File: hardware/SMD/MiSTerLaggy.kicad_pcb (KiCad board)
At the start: 2 copper layers, 19.8 x 12.5 mm, 9 parts, among them J1 USB_C_Receptacle_USB2.0, Q1 Q_Photo_NPN

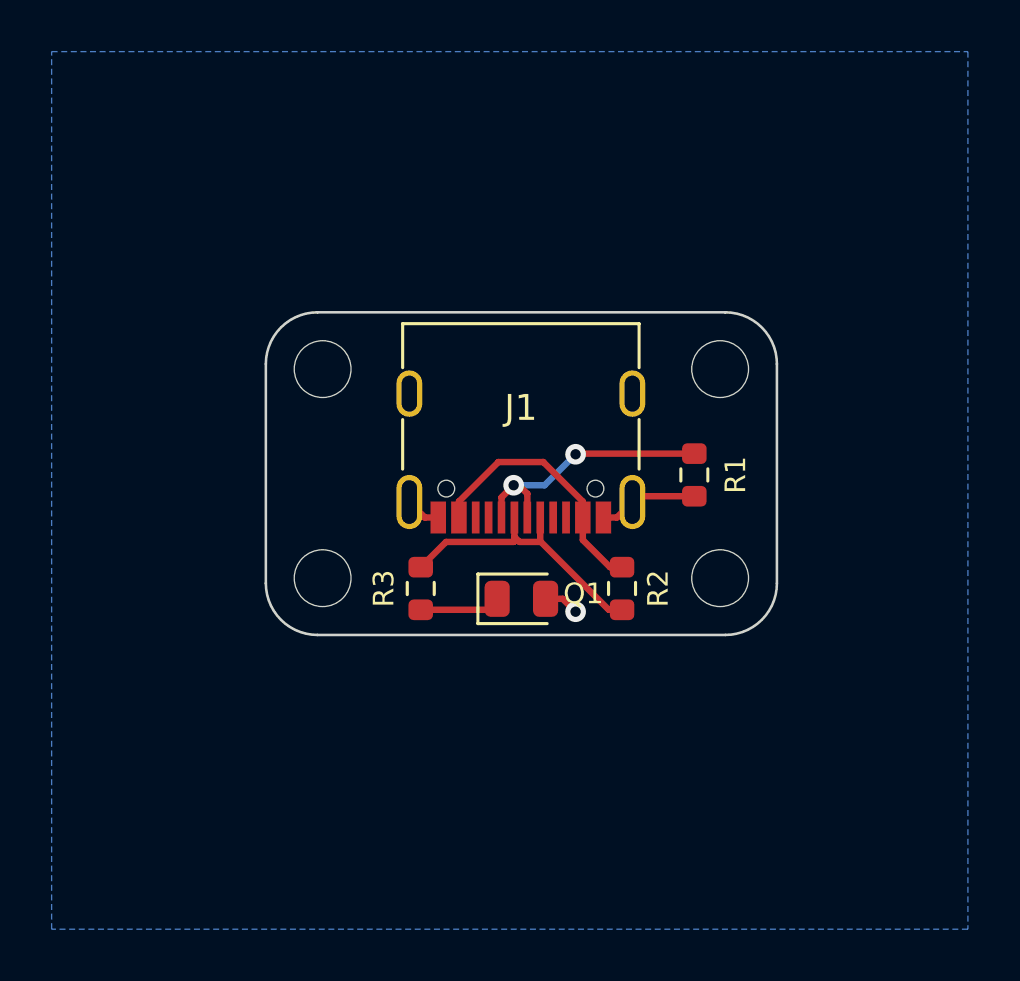
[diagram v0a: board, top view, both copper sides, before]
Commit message: New circuit design
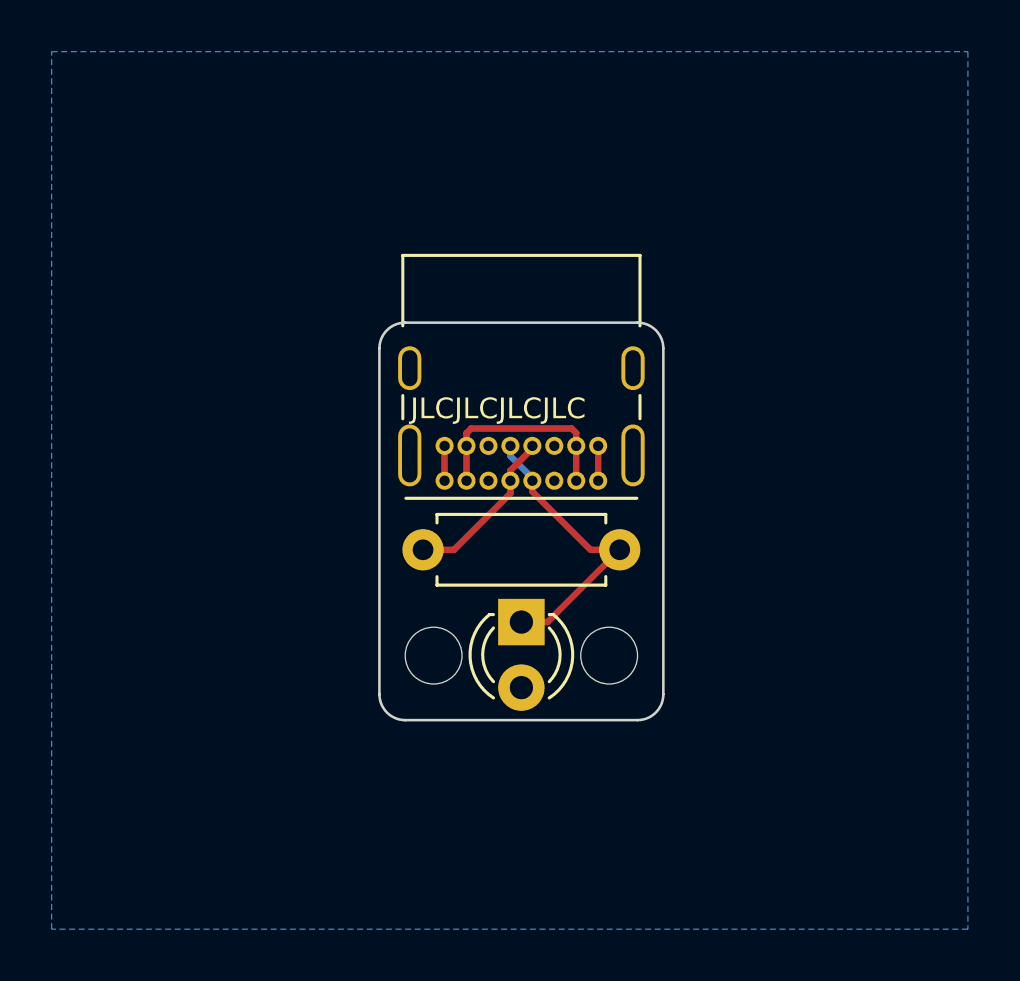
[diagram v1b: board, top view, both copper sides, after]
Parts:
- removed H3, H4: MountingHole_Pad, MountingHole:MountingHole_2.2mm_M2_ISO7380
- removed the R1 at (134.4, 73.4)
- removed R2: ??, Resistor_SMD:R_0603_1608Metric
- J1: footprint Connector_USB:USB_C_Receptacle_G-Switch_GT-USB-7010ASV -> Connector_USB:USB_C_Receptacle_GCT_USB4085
- Q1: value Q_Photo_NPN -> PT17-21C/L41/TR8; footprint LED_SMD:LED_0805_2012Metric -> LED_THT:LED_D3.0mm
- R1: renamed from R3; value ?? -> 750K; footprint Resistor_SMD:R_0603_1608Metric -> Resistor_THT:R_Axial_DIN0207_L6.3mm_D2.5mm_P7.62mm_Horizontal
- moved H2 11.9 mm to (131.1, 80.4)
- moved H1 11.9 mm to (124.3, 80.4)
- moved R1 7.85 mm to (131.5, 76.3), turned to 180 degrees
- moved J1 3.78 mm to (130.7, 73.6)
- moved Q1 0.90 mm to (127.7, 79.1), turned to -90 degrees
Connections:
- net Net-(J1-D--PadA7) renamed +3.3V
- J1 pad A4: +5V -> unconnected-(J1-VBUS-PadA4)
- J1 pad A6: Net-(J1-D+-PadA6) -> Net-(Q1-C)
- J1 pad A9: +5V -> unconnected-(J1-VBUS-PadA4)
- J1 pad B4: +5V -> unconnected-(J1-VBUS-PadA4)
- J1 pad B6: Net-(J1-D+-PadA6) -> Net-(Q1-C)
- J1 pad B9: +5V -> unconnected-(J1-VBUS-PadA4)
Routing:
- net Net-(J1-D+-PadA6): track 10.5 -> 0.00 mm, vias 2 -> 0
- net +5V: track 10.1 -> 0.00 mm
- net Net-(Q1-C): track 3.14 -> 11.4 mm
- net unconnected-(J1-VBUS-PadA4): track 0.00 -> 8.09 mm
- net +3.3V: track 11.2 -> 6.49 mm
- net GND: track 6.60 -> 2.70 mm, vias 1 -> 0
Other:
- board size 19.8 x 12.5 mm -> 11 x 15.4 mm
- board text added: "@wickerwaka"
- board text added: "JLCJLCJLCJLC"
- board text added: "MrLaggy"
- board text added: "v1.0"

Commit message: MOSFET usage
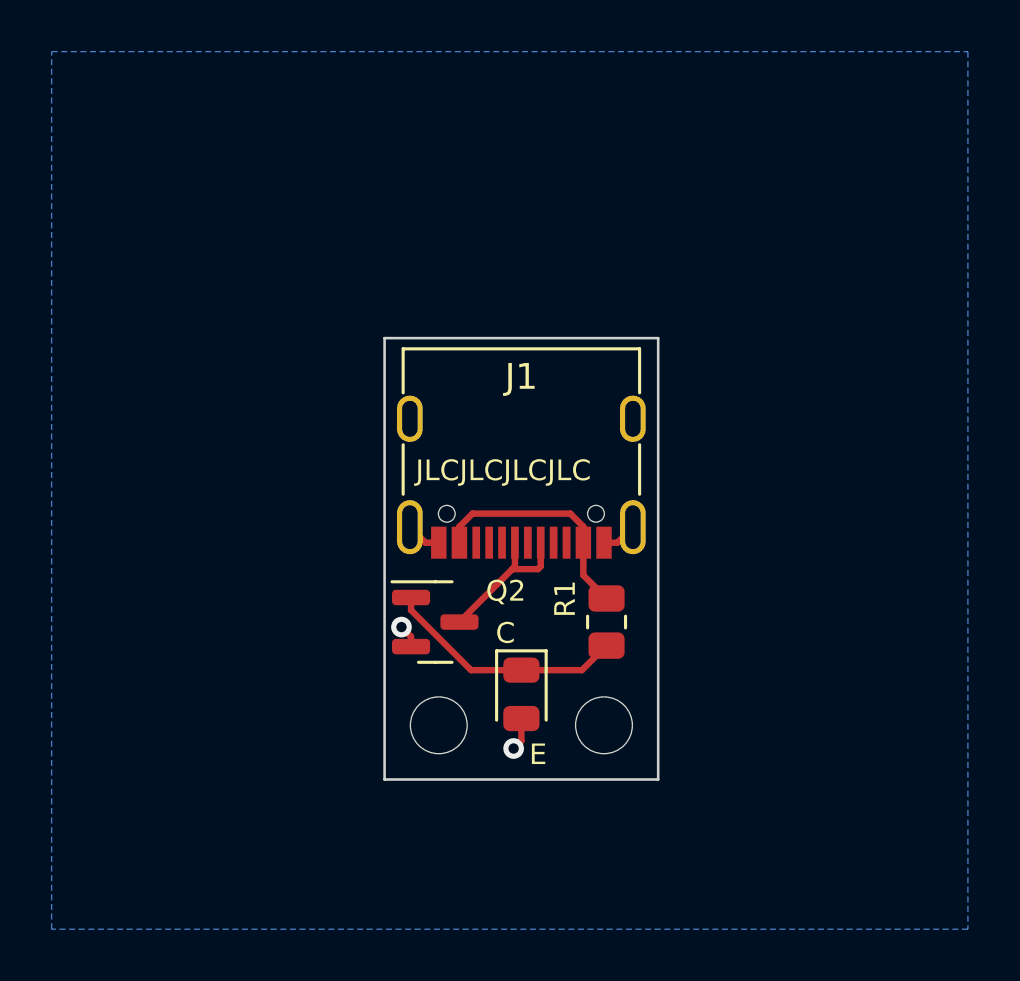
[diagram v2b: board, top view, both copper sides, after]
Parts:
- added Q2: 2N7002, Package_TO_SOT_SMD:SOT-23, F.Cu at (124.4, 79.1)
- J1: footprint Connector_USB:USB_C_Receptacle_GCT_USB4085 -> Connector_USB:USB_C_Receptacle_G-Switch_GT-USB-7010ASV
- Q1: footprint LED_THT:LED_D3.0mm -> LED_SMD:LED_0805_2012Metric
- R1: footprint Resistor_THT:R_Axial_DIN0207_L6.3mm_D2.5mm_P7.62mm_Horizontal -> Resistor_SMD:R_0805_2012Metric
- moved J1 3.26 mm to (127.7, 72.3)
- moved R1 2.85 mm to (131.0, 79.1), turned to 90 degrees
- moved Q1 2.80 mm to (127.7, 81.9)
- moved H1 2.71 mm to (124.5, 83.1)
- moved H2 2.71 mm to (130.9, 83.1)
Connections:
- J1 pad A4: unconnected-(J1-VBUS-PadA4) -> Net-(J1-VBUS-PadA4)
- J1 pad A6: Net-(Q1-C) -> unconnected-(J1-D+-PadA6)
- J1 pad A7: +3.3V -> Net-(Q2-D)
- J1 pad A9: unconnected-(J1-VBUS-PadA4) -> Net-(J1-VBUS-PadA4)
- J1 pad B4: unconnected-(J1-VBUS-PadA4) -> Net-(J1-VBUS-PadA4)
- J1 pad B6: Net-(Q1-C) -> unconnected-(J1-D+-PadB6)
- J1 pad B7: +3.3V -> Net-(Q2-D)
- J1 pad B9: unconnected-(J1-VBUS-PadA4) -> Net-(J1-VBUS-PadA4)
- R1 pad 2: +3.3V -> Net-(J1-VBUS-PadA4)
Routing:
- net Net-(J1-VBUS-PadA4): track 0.00 -> 8.99 mm
- net unconnected-(J1-VBUS-PadA4): track 8.09 -> 0.00 mm
- net +3.3V: track 6.49 -> 0.00 mm
- net Net-(Q2-D): track 0.00 -> 6.03 mm
- net GND: track 2.70 -> 4.93 mm, vias 0 -> 2
- net Net-(Q1-C): track 11.4 -> 9.42 mm
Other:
- board size 11 x 15.4 mm -> 10.6 x 17.1 mm
- board text added: "C"
- board text added: "E"
